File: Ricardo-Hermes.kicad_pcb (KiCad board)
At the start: 4 copper layers, 42.8 x 63.6 mm, 145 parts, among them IC2 SX1280, J1 RBUS, J2 USB_C_Receptacle_USB2.0, J3 Conn_01x03_Pin, J4 Conn_01x03_Pin, U1 ESP32-S3, U11 SC4215ASTRT, U12 SKY66112-11, U13 DEA202450BT-1213C1, U2 SN65HVD230, U3 LM66200DRLR, U4 MAX77827AEFD+T, U5 SC4215ASTRT, U6 DEA202450BT-1213C1, Y1 R940000171, Y3 Crystal_GND24

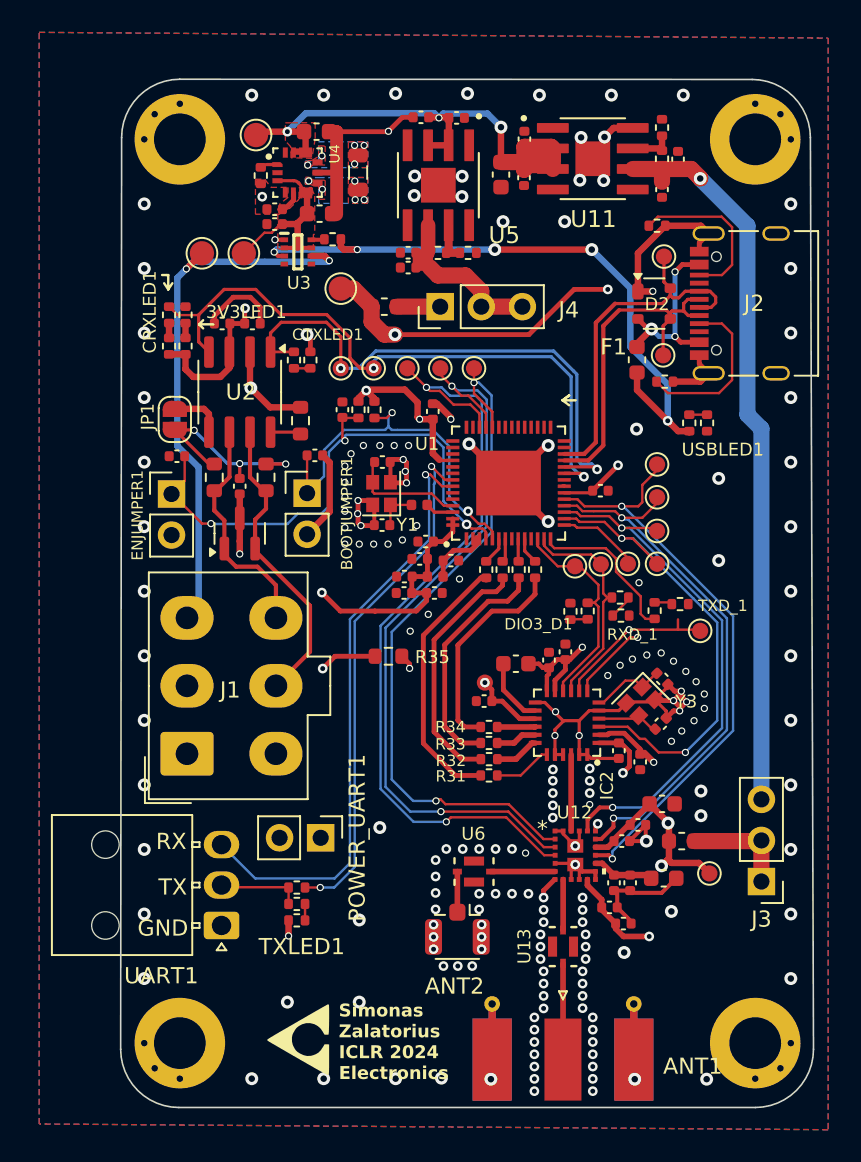
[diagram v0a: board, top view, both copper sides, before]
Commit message: Tidying up
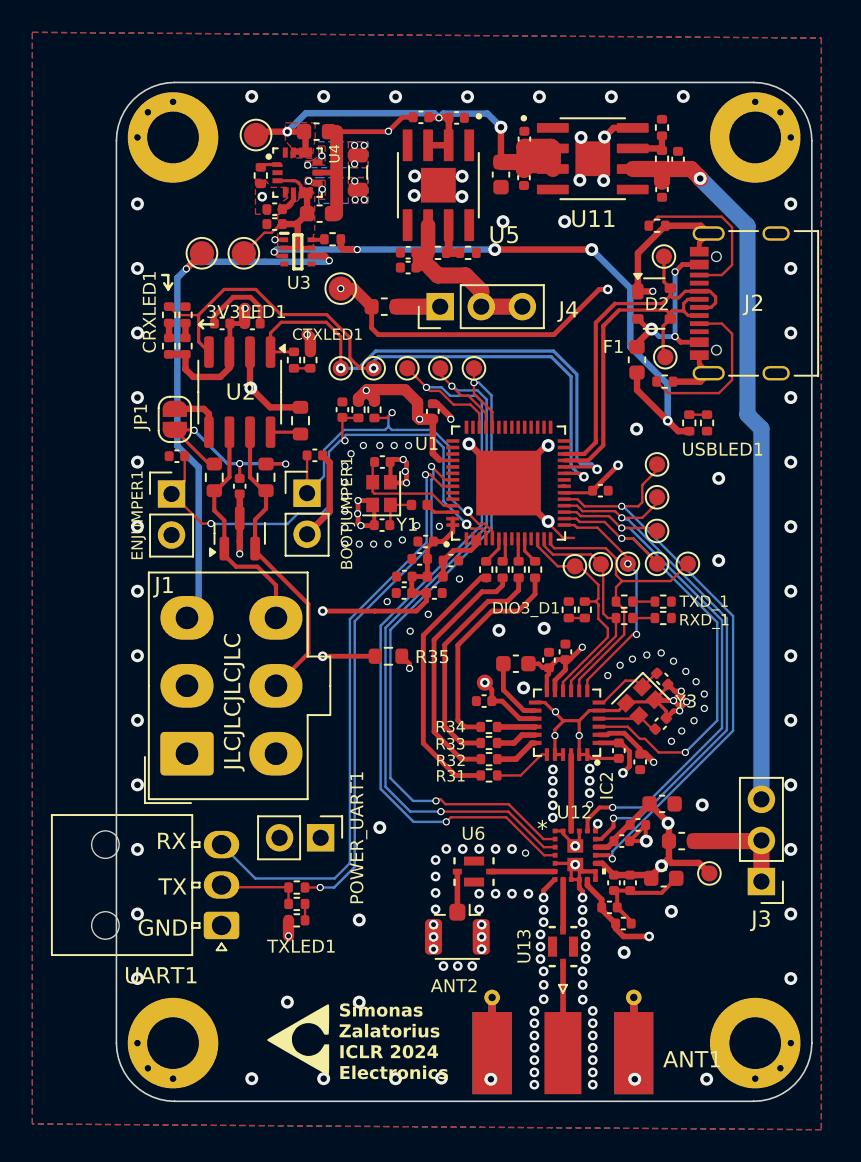
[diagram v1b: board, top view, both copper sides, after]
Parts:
- moved DIO1 4.21 mm to (153.5, 101.0)
- moved RXD_1 2.62 mm to (152.0, 104.3)
- moved R36 1.96 mm to (149.6, 103.3), turned to 0 degrees
- moved R37 1.30 mm to (149.6, 104.3)
- moved TXD_1 1.05 mm to (152.0, 103.3)
- moved H1 0.44 mm to (121.7, 74.6)
- moved H3 0.42 mm to (121.7, 130.6)
- moved ANT1 0.40 mm to (145.8, 129.5)
- moved R38 0.19 mm to (147.2, 103.8)
- moved D-_TP1 0.18 mm to (152.1, 88.2)
- moved DIO3_D1 0.14 mm to (146.2, 103.8)
- moved H2 0.12 mm to (157.7, 74.6)
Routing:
- net SX_BUSY: track 10.0 -> 14.6 mm, vias 1 -> 2
- net GND: track 326.9 -> 330.7 mm, vias 200 -> 201
- net +3V3: track 131.5 -> 128.9 mm
- net VAA: track 50.0 -> 51.0 mm
- net DIO1: track 19.9 -> 19.1 mm, vias 1 -> 0
- net DIO3: track 13.3 -> 14.0 mm
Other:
- board size 42.8 x 63.6 mm -> 43 x 63 mm
- board text added: "JLCJLCJLCJLC"
